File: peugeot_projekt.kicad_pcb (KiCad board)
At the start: 2 copper layers, 65 x 58.3 mm, 27 parts, among them J1 ESP Power selector, J2 +12V Permanent, J3 Main Power and Data, J4 LCD Power, P1 Conn_02x20_Odd_Even, U1 ESP32, U2 LevelShifter4Shield, U3 TSS463C, U4 MCP2551-I-SN, U5 LM7805_TO220, Y1 8MHz

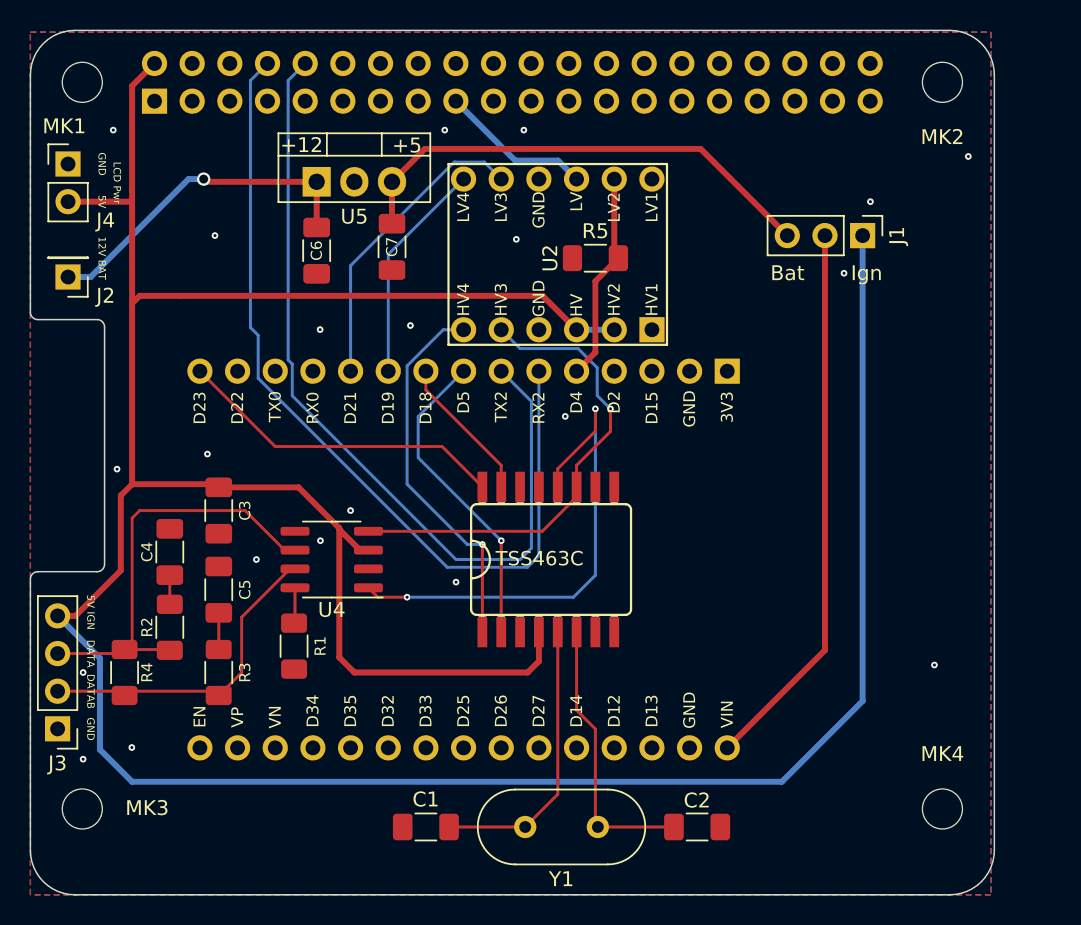
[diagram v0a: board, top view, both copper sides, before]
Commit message: Progress on v0.2 of the board
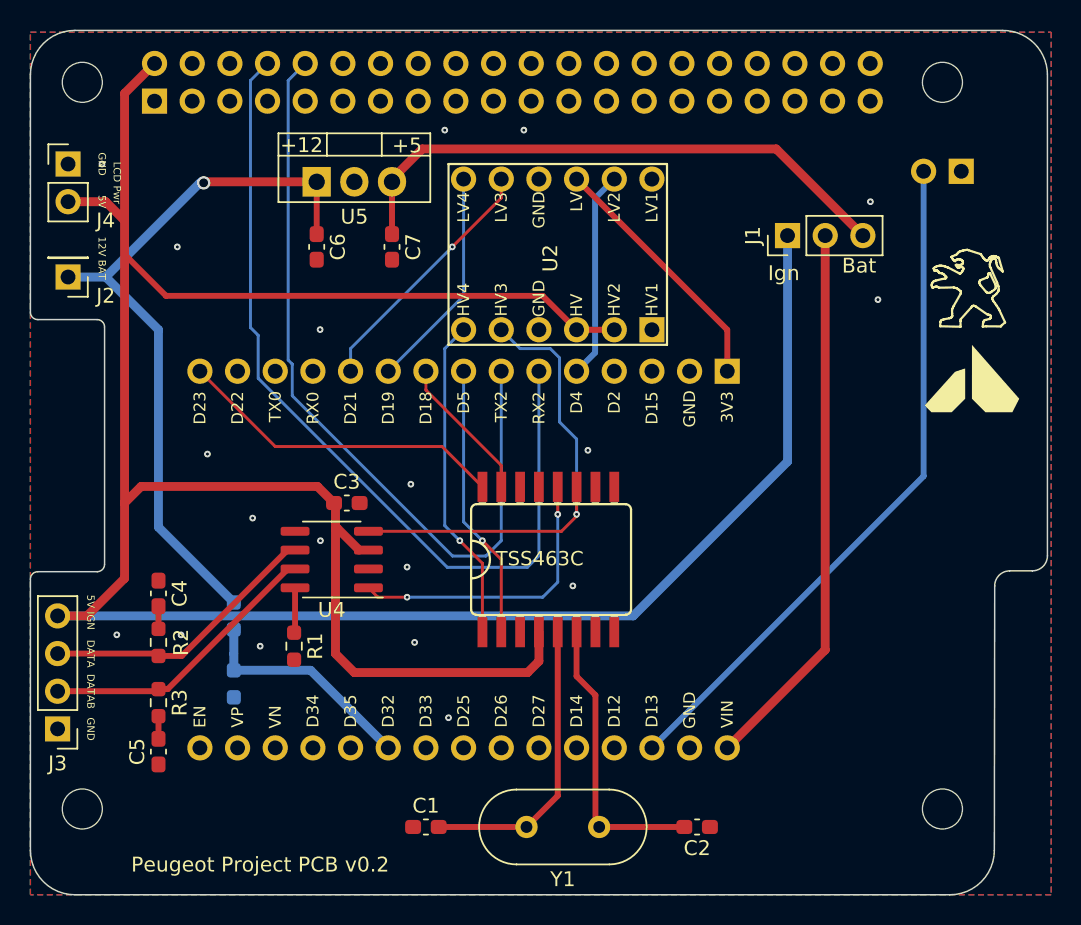
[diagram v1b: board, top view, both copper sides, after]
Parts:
- removed R4: 120, Resistor_SMD:R_1206_3216Metric_Pad1.30x1.75mm_HandSolder
- added G***: LOGO, lib:orqa_logo, F.Cu at (263.5, 117.5)
- added G***: LOGO, lib:peugeot_logo, F.Cu at (263.2, 111.4)
- added J7: RUN Header 3B, Connector_PinSocket_2.54mm:PinSocket_1x02_P2.54mm_Vertical, B.Cu at (262.8, 103.5)
- added R6: 10k, Resistor_SMD:R_0603_1608Metric_Pad0.98x0.95mm_HandSolder, B.Cu at (213.7, 138.1)
- C1, C2, C3, C4, C5, C6, C7: footprint Capacitor_SMD:C_1206_3216Metric_Pad1.33x1.80mm_HandSolder -> Capacitor_SMD:C_0603_1608Metric_Pad1.08x0.95mm_HandSolder
- R1, R2, R3: footprint Resistor_SMD:R_1206_3216Metric_Pad1.30x1.75mm_HandSolder -> Resistor_SMD:R_0603_1608Metric_Pad0.98x0.95mm_HandSolder
- R5: value 10k -> 100k; footprint Resistor_SMD:R_1206_3216Metric_Pad1.30x1.75mm_HandSolder -> Resistor_SMD:R_0603_1608Metric_Pad0.98x0.95mm_HandSolder; moved to B.Cu
- moved R5 34.3 mm to (213.7, 133.5), turned to -90 degrees
- moved C5 11.7 mm to (208.6, 142.6), turned to 90 degrees
- moved C3 8.65 mm to (221.3, 125.9), turned to 0 degrees
- moved J1 5.07 mm to (251.1, 107.8), turned to 90 degrees
- moved R3 4.54 mm to (208.6, 139.3), turned to -90 degrees
- moved C4 2.90 mm to (208.6, 132.0)
- moved R2 1.27 mm to (208.6, 135.3)
- moved C6 0.25 mm to (219.3, 108.6)
- moved Y1 0.09 mm to (238.4, 147.7)
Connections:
- R5 pad 1: GNDD -> Net-(C6-Pad1)
- R5 pad 2: /Wake PIN -> /Voltmeter
- U1 pad 13: unconnected-(U1-Pad13) -> /RUN
- U1 pad 30: unconnected-(U1-Pad30) -> /3V3 - LVL_SHFT
- U1 pad 6: unconnected-(U1-Pad6) -> /Voltmeter
- U2 pad 3: +3V3 -> /3V3 - LVL_SHFT
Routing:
- net /RUN: track 0.00 -> 46.5 mm
- net Net-(C6-Pad1): track 22.9 -> 48.5 mm
- net +5V: track 217.4 -> 193.4 mm
- net /3V3 - LVL_SHFT: track 0.00 -> 17.2 mm
- net /Voltmeter: track 0.00 -> 15.3 mm
- net /VAN_TX: track 33.7 -> 19.9 mm
- net +3V3: track 10.3 -> 0.00 mm
- net /DATA: track 28.8 -> 18.5 mm
- net /+5V permanent: track 32.8 -> 38.5 mm
- net /MISO: track 24.8 -> 21.3 mm
- net Net-(U1-Pad20): track 20.6 -> 17.2 mm, vias 0 -> 1
- net /GPIO15(RXD0): track 56.8 -> 53.4 mm
- net /SS: track 20.5 -> 18.0 mm
- net /DATAB: track 21.4 -> 19.4 mm
- net /VAN_RX: track 32.6 -> 31.5 mm
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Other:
- board size 65 x 58.3 mm -> 68.6 x 58.3 mm
- board text added: "Peugeot Project PCB v0.2"
